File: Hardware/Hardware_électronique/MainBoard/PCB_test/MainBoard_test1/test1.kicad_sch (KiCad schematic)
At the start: 17 parts, among them J1 Conn_RasPi, Q1 PMOS

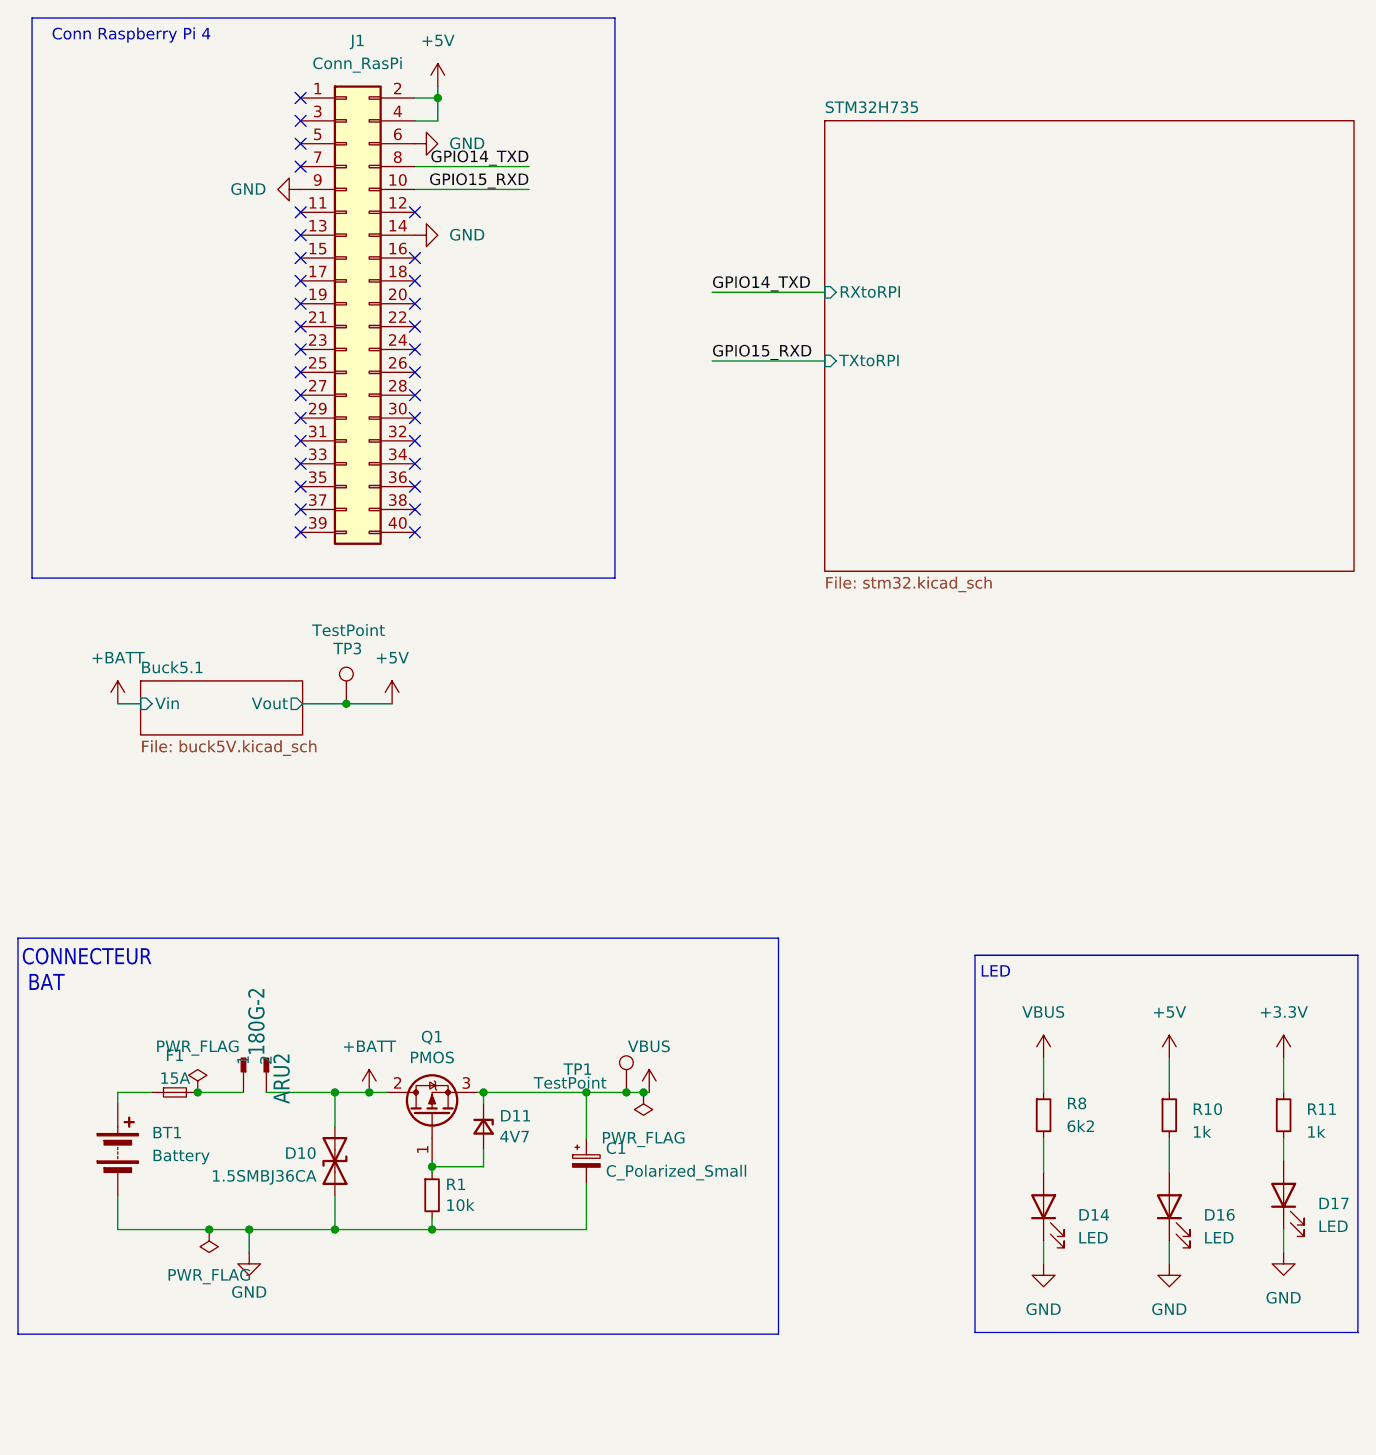
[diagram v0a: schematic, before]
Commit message: quite finished schematics
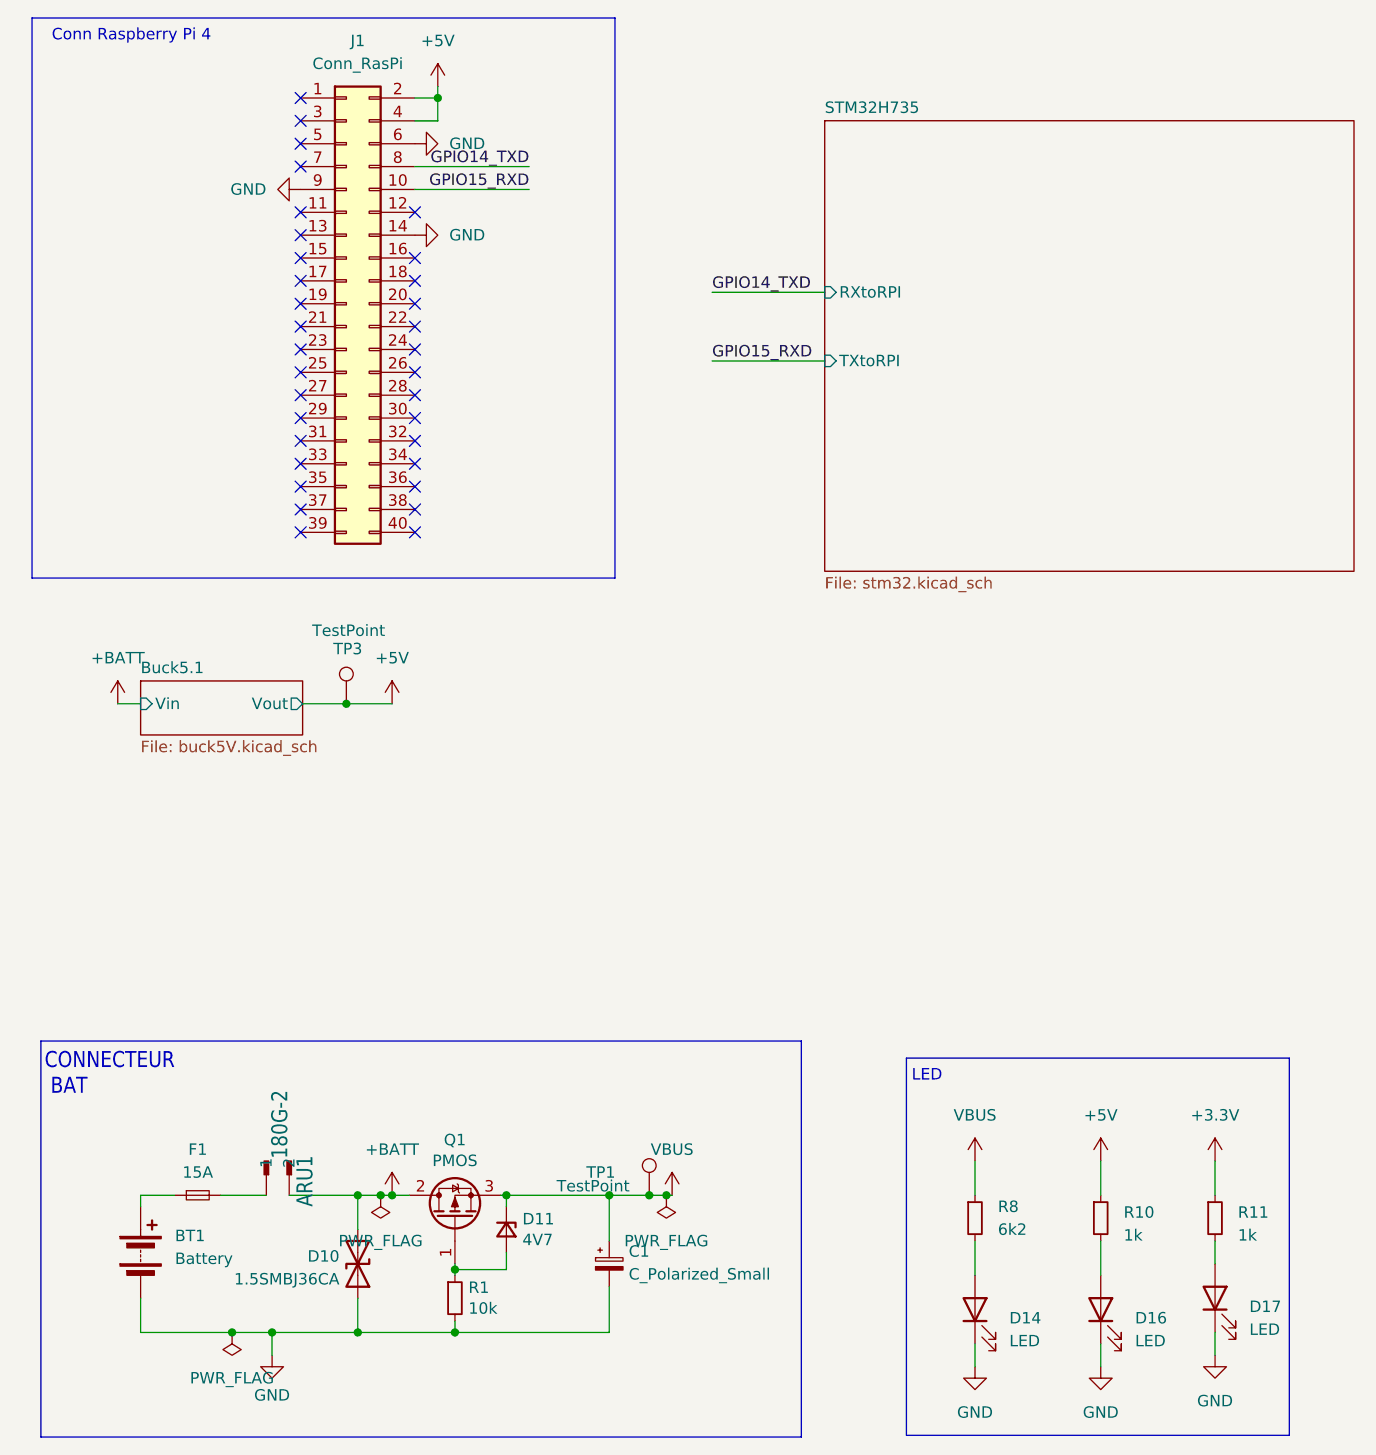
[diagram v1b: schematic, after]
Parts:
- removed ARU2: 180G-2, MainBoard:180G-2, symbol schematic1-eagle-import:180G-2
- added ARU1: 180G-2, MainBoard:180G-2, symbol schematic1-eagle-import:180G-2
- F1: footprint Fuse:Fuse_1206_3216Metric_Pad1.42x1.75mm_HandSolder -> (none); Mouser Part Number 693-3413.0330.22 -> (none)
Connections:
- net +BATT: now also ARU1.2
- net at F1.2: now also ARU1.1
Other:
- moved on the sheet: D14, D16, D17, R10, R11, R8
